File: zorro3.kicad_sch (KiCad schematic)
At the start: 5 parts, among them CN1 Zorro3, U1 CY74FCT16543TPVCT, U2 CY74FCT16543TPVCT, U3 CY74FCT16543TPVCT, U5 CY74FCT543ATQCT

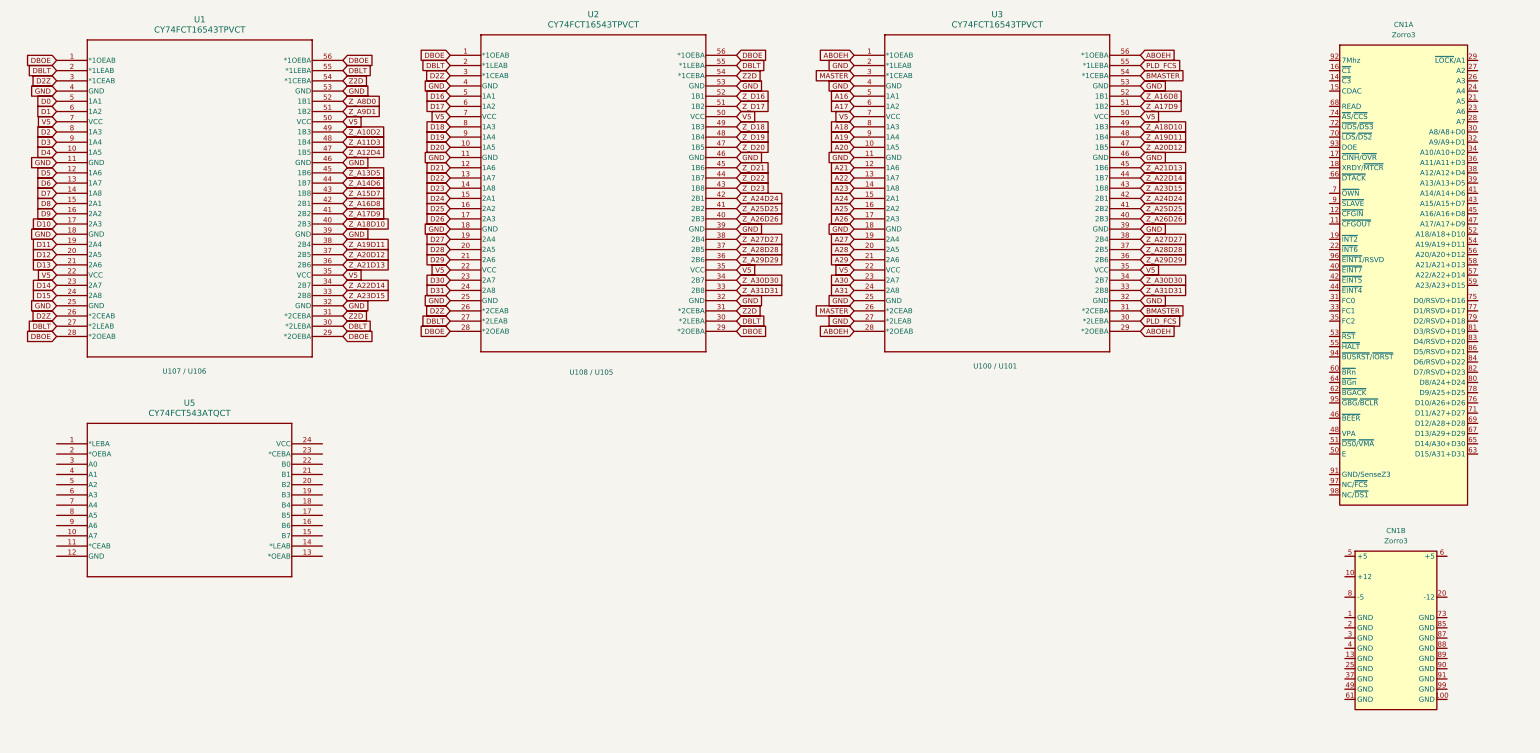
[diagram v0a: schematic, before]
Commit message: Update design
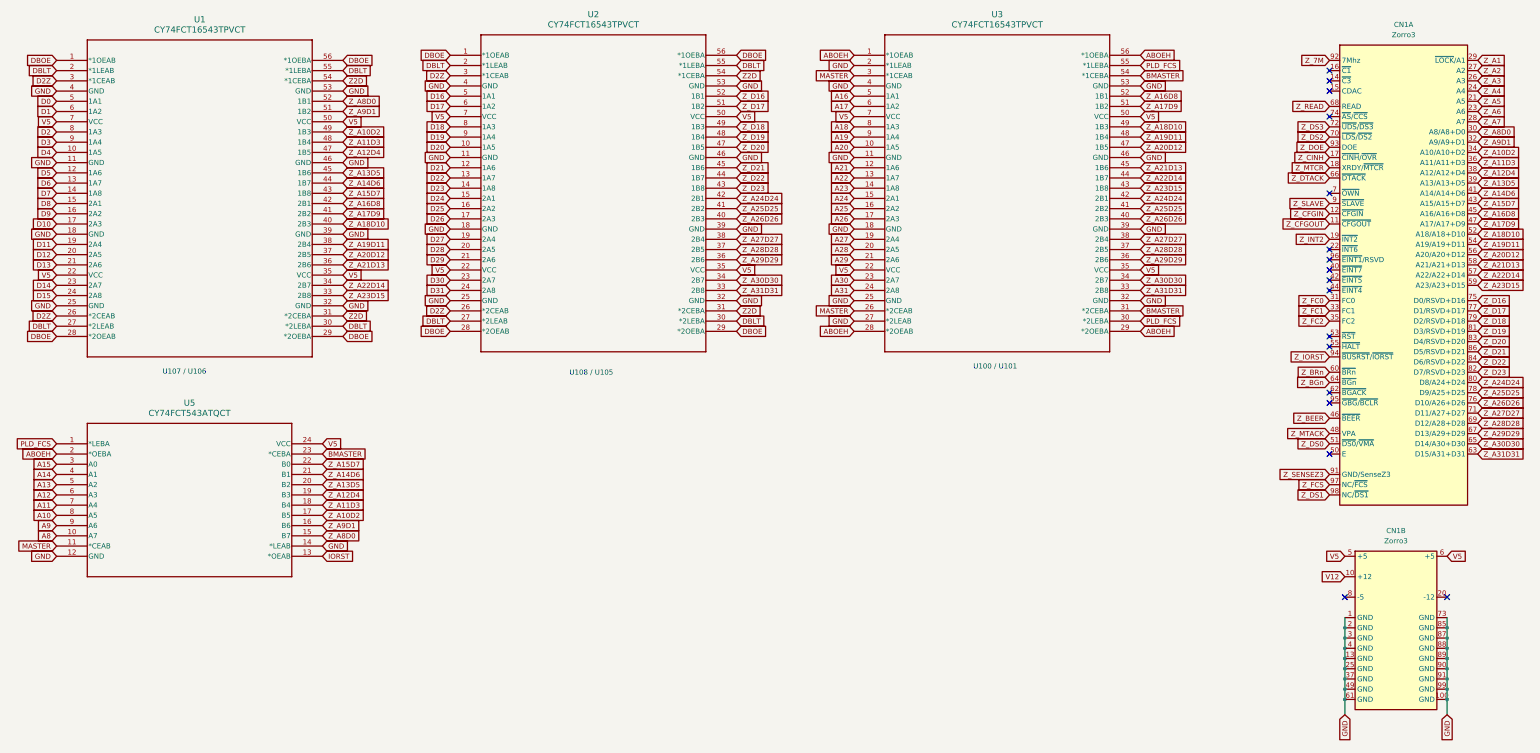
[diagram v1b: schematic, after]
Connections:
- net ABOEH: now also U5.2 (*OEBA)
- net BMASTER: now also U5.23 (*CEBA)
- net GND: now also CN1.1 (GND), CN1.100 (GND), CN1.13 (GND), CN1.2 (GND), CN1.25 (GND), CN1.3 (GND), CN1.37 (GND), CN1.4 (GND), CN1.49 (GND), CN1.61 (GND), CN1.73 (GND), CN1.85 (GND), CN1.87 (GND), CN1.88 (GND), CN1.89 (GND), CN1.90 (GND), CN1.91 (GND), CN1.99 (GND), U5.12 (GND), U5.14 (*LEAB)
- net MASTER: now also U5.11 (*CEAB)
- net PLD_FCS: now also U5.1 (*LEBA)
- net V5: now also CN1.5 (+5), CN1.6 (+5), U5.24 (VCC)
- net Z_A10D2: now also CN1.34 (A10/A10+D2), U5.17 (B5)
- net Z_A11D3: now also CN1.36 (A11/A11+D3), U5.18 (B4)
- net Z_A12D4: now also CN1.38 (A12/A12+D4), U5.19 (B3)
- net Z_A13D5: now also CN1.39 (A13/A13+D5), U5.20 (B2)
- net Z_A14D6: now also CN1.41 (A14/A14+D6), U5.21 (B1)
- net Z_A15D7: now also CN1.43 (A15/A15+D7), U5.22 (B0)
- net Z_A16D8: now also CN1.45 (A16/A16+D8)
- net Z_A17D9: now also CN1.47 (A17/A17+D9)
- net Z_A18D10: now also CN1.52 (A18/A18+D10)
- net Z_A19D11: now also CN1.54 (A19/A19+D11)
- net Z_A20D12: now also CN1.56 (A20/A20+D12)
- net Z_A21D13: now also CN1.58 (A21/A21+D13)
- net Z_A22D14: now also CN1.57 (A22/A22+D14)
- net Z_A23D15: now also CN1.59 (A23/A23+D15)
- net Z_A24D24: now also CN1.80 (D8/A24+D24)
- net Z_A25D25: now also CN1.78 (D9/A25+D25)
- net Z_A26D26: now also CN1.76 (D10/A26+D26)
- net Z_A27D27: now also CN1.71 (D11/A27+D27)
- net Z_A28D28: now also CN1.69 (D12/A28+D28)
- net Z_A29D29: now also CN1.67 (D13/A29+D29)
- net Z_A30D30: now also CN1.65 (D14/A30+D30)
- net Z_A31D31: now also CN1.63 (D15/A31+D31)
- net Z_A8D0: now also CN1.30 (A8/A8+D0), U5.15 (B7)
- net Z_A9D1: now also CN1.32 (A9/A9+D1), U5.16 (B6)
- net Z_D16: now also CN1.75 (D0/RSVD+D16)
- net Z_D17: now also CN1.77 (D1/RSVD+D17)
- net Z_D18: now also CN1.79 (D2/RSVD+D18)
- net Z_D19: now also CN1.81 (D3/RSVD+D19)
- net Z_D20: now also CN1.83 (D4/RSVD+D20)
- net Z_D21: now also CN1.86 (D5/RSVD+D21)
- net Z_D22: now also CN1.84 (D6/RSVD+D22)
- net Z_D23: now also CN1.82 (D7/RSVD+D23)
- net A8: now reaches U5.10 (A7)
- net IORST: now reaches U5.13 (*OEAB)
- net A15: now reaches U5.3 (A0)
- net A14: now reaches U5.4 (A1)
- net A13: now reaches U5.5 (A2)
- net A12: now reaches U5.6 (A3)
- net A11: now reaches U5.7 (A4)
- net A10: now reaches U5.8 (A5)
- net A9: now reaches U5.9 (A6)
- net Z_CFGOUT: now reaches CN1.11 (~{CFGOUT})
- net Z_CFGIN: now reaches CN1.12 (~{CFGIN})
- net Z_CINH: now reaches CN1.17 (~{CINH}/~{OVR})
- net Z_MTCR: now reaches CN1.18 (XRDY/~{MTCR})
- net Z_INT2: now reaches CN1.19 (~{INT2})
- net Z_A5: now reaches CN1.21 (A5)
- net Z_A6: now reaches CN1.23 (A6)
- net Z_A4: now reaches CN1.24 (A4)
- net Z_A3: now reaches CN1.26 (A3)
- net Z_A2: now reaches CN1.27 (A2)
- net Z_A7: now reaches CN1.28 (A7)
- net Z_A1: now reaches CN1.29 (~{LOCK}/A1)
- net Z_FC0: now reaches CN1.31 (FC0)
- net Z_FC1: now reaches CN1.33 (FC1)
- net Z_FC2: now reaches CN1.35 (FC2)
- net Z_BEER: now reaches CN1.46 (~{BEER})
- net Z_MTACK: now reaches CN1.48 (VPA)
- net Z_DS0: now reaches CN1.51 (~{DS0}/~{VMA})
- net Z_BRn: now reaches CN1.60 (~{BRn})
- net Z_BGn: now reaches CN1.64 (~{BGn})
- net Z_DTACK: now reaches CN1.66 (~{DTACK})
- net Z_READ: now reaches CN1.68 (READ)
- net Z_DS2: now reaches CN1.70 (~{LDS}/~{DS2})
- net Z_DS3: now reaches CN1.72 (~{UDS}/~{DS3})
- net Z_SLAVE: now reaches CN1.9 (~{SLAVE})
- net Z_SENSEZ3: now reaches CN1.91 (GND/SenseZ3)
- net Z_7M: now reaches CN1.92 (7Mhz)
- net Z_DOE: now reaches CN1.93 (DOE)
- net Z_IORST: now reaches CN1.94 (~{BUSRST}/~{IORST})
- net Z_FCS: now reaches CN1.97 (NC/~{FCS})
- net Z_DS1: now reaches CN1.98 (NC/~{DS1})
- net V12: now reaches CN1.10 (+12)
- no-connect marks 0 -> 17

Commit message: More work. Getting there.
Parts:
- added C5: 10pF, symbol Device:C_Small
- added R12, R13, R14, R15, R16: 1K, YC324-FK-071KL:RESCAXS127P508X320X70-8N, symbol YC324-FK-071KL:YC324-FK-071KL
- added U11: SN74ABT16374ADGGR, DGG48, symbol SN74ABT16374ADGGR:SN74ABT16374ADGGR
- added U12: 74LVC07APW_118, TSSOP14_5P1X4P5_NEX, symbol 74LVC07APW_118:74LVC07APW_118
- added U13: SN74ABT16245ADGGR, DGG48, symbol SN74ABT16245ADGGR:SN74ABT16245ADGGR
- added U14: 74ACT521MTCX, TSSOP20_4P4X6P5_ONS, symbol 74ACT521MTCX:74ACT521MTCX
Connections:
- net A24: now also U14.17 (A7)
- net A25: now also U14.15 (A6)
- net A26: now also U14.13 (A5)
- net A27: now also U14.11 (A4)
- net A28: now also U14.8 (A3)
- net A29: now also U14.6 (A2)
- net A30: now also U14.4 (A1)
- net A31: now also U14.2 (A0)
- net BMASTER: now also U13.1 (1DIR), U13.24 (2DIR)
- net D0: now also U11.26 (2D8)
- net D1: now also U11.22 (2Q7), U11.23 (2Q8), U11.27 (2D7)
- net D2: now also U11.20 (2Q6), U11.29 (2D6)
- net D24: now also U11.37 (1D8)
- net D25: now also U11.38 (1D7)
- net D26: now also U11.40 (1D6)
- net D27: now also U11.41 (1D5)
- net D28: now also U11.43 (1D4)
- net D29: now also U11.44 (1D3)
- net D3: now also U11.19 (2Q5), U11.30 (2D5)
- net D30: now also U11.46 (1D2)
- net D31: now also U11.47 (1D1)
- net D4: now also U11.17 (2Q4), U11.32 (2D4)
- net D5: now also U11.16 (2Q3), U11.33 (2D3)
- net D6: now also U11.14 (2Q2), U11.35 (2D2)
- net D7: now also U11.13 (2Q1), U11.36 (2D1)
- net GND: now also C5.2, R16.5, U11.10 (GND), U11.15 (GND), U11.21 (GND), U11.28 (GND), U11.34 (GND), U11.39 (GND), U11.4 (GND), U11.45 (GND), U12.11 (5A), U12.13 (6A), U12.7 (GND), U13.10 (GND), U13.15 (GND), U13.21 (GND), U13.28 (GND), U13.34 (GND), U13.39 (GND), U13.4 (GND), U13.45 (GND), U14.1 (*IA=B), U14.10 (GND)
- net IORST: now also U12.8 (4Y)
- net V5: now also R12.5, R12.6, R12.7, R12.8, R13.5, R13.6, R13.7, R13.8, R14.5, R14.6, R14.7, R14.8, R15.5, R15.6, R15.7, R15.8, R16.7, R16.8, U11.18 (VCC), U11.31 (VCC), U11.42 (VCC), U11.7 (VCC), U12.14 (VCC), U13.18 (VCC), U13.31 (VCC), U13.42 (VCC), U13.7 (VCC), U14.20 (VCC)
- net Z_A2: now also U13.9 (1B6)
- net Z_A3: now also U13.8 (1B5)
- net Z_A4: now also U13.6 (1B4)
- net Z_A5: now also U13.5 (1B3)
- net Z_A6: now also U13.3 (1B2)
- net Z_A7: now also U13.2 (1B1)
- net Z_CFGOUT: now also U11.1 (*1OE)
- net Z_DOE: now also U13.16 (2B3)
- net Z_DS0: now also U13.23 (2B8)
- net Z_DS1: now also U13.22 (2B7)
- net Z_DS2: now also U13.20 (2B6)
- net Z_DS3: now also U13.19 (2B5)
- net Z_DTACK: now also C5.1
- net Z_FC0: now also U13.14 (2B2)
- net Z_FC1: now also U13.13 (2B1)
- net Z_FC2: now also U13.11 (1B7)
- net Z_IORST: now also U12.9 (4A)
- net Z_MTCR: now also U13.17 (2B4)
- net Z_READ: now also U13.12 (1B8)
- new net A2: U13.40 (1A6)
- new net A3: U13.41 (1A5)
- new net A4: U13.43 (1A4)
- new net A5: U13.44 (1A3)
- new net A6: U13.46 (1A2)
- new net A7: U13.47 (1A1)
- new net ABOEL: U13.25 (*2OE), U13.48 (*1OE)
- new net BERR: U12.6 (3Y)
- new net LED: U12.2 (1Y), U12.4 (2Y)
- new net M24: R12.1, U11.12 (1Q8), U14.18 (B7)
- new net M25: R12.2, U11.11 (1Q7), U14.16 (B6)
- new net M26: R12.3, U11.9 (1Q6), U14.14 (B5)
- new net M27: R12.4, U11.8 (1Q5), U14.12 (B4)
- new net M28: R13.1, U11.6 (1Q4), U14.9 (B4)
- new net M29: R13.2, U11.5 (1Q3), U14.7 (B2)
- new net M30: R13.3, U11.3 (1Q2), U14.5 (B1)
- new net M31: R13.4, U11.2 (1Q1), U14.3 (B0)
- new net MATCH: U14.19 (*OA=B)
- new net PLD_CFGLT: U11.48 (1CLK)
- new net PLD_DOE: R16.4, U13.33 (2A3)
- new net PLD_DS0: R15.4
- new net PLD_DS1: R15.3, U13.26 (2A8), U13.27 (2A7)
- new net PLD_DS2: R15.2, U13.29 (2A6)
- new net PLD_DS3: R15.1, U13.30 (2A5)
- new net PLD_FC0: R14.4, U13.35 (2A2)
- new net PLD_FC1: R14.3, U13.36 (2A1)
- new net PLD_FC2: R14.1, U13.38 (1A7)
- new net PLD_INTREG: U11.25 (2CLK)
- new net PLD_INTVEC: U11.24 (*2OE)
- new net PLD_MTCR: R16.1, U13.32 (2A4)
- new net PLD_READ: R14.2, U13.37 (1A8)
- new net SCSI_BUSY: U12.1 (1A), U12.3 (2A)
- new net Z_BERR: U12.5 (3A)
- new net Z_SENSE3: R16.2
- no-connect marks 17 -> 22
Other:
- note added: "2x8bit register w/ 3state"
- note added: "Identity Comparator"
- note added: "Is this intentional?"
- note added: "TODO 1x374 + 521 move into CPLD"
- note added: "USE 74ABT16543 instead of 74FCT16543"
- note added: "Z_DS3 + Z_DS2 have FBs on original but not Z_DS1 and Z_DS0"
- moved on the sheet: CN1A, CN1B
